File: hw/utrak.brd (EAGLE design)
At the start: 15.9 x 49.8 mm, 46 parts, among them IC1 SI4060, Q1 BLAH, U1 TLV61225

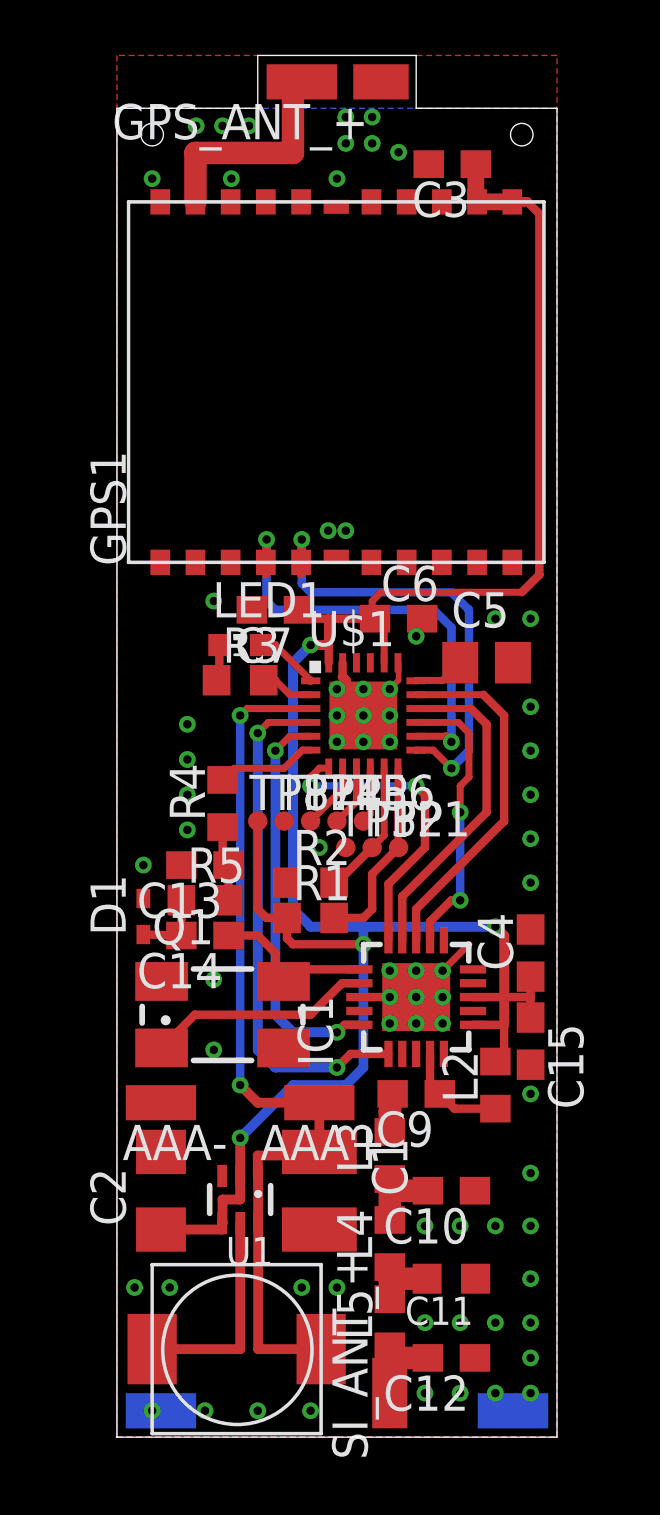
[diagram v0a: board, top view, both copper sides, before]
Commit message: add new hardware files
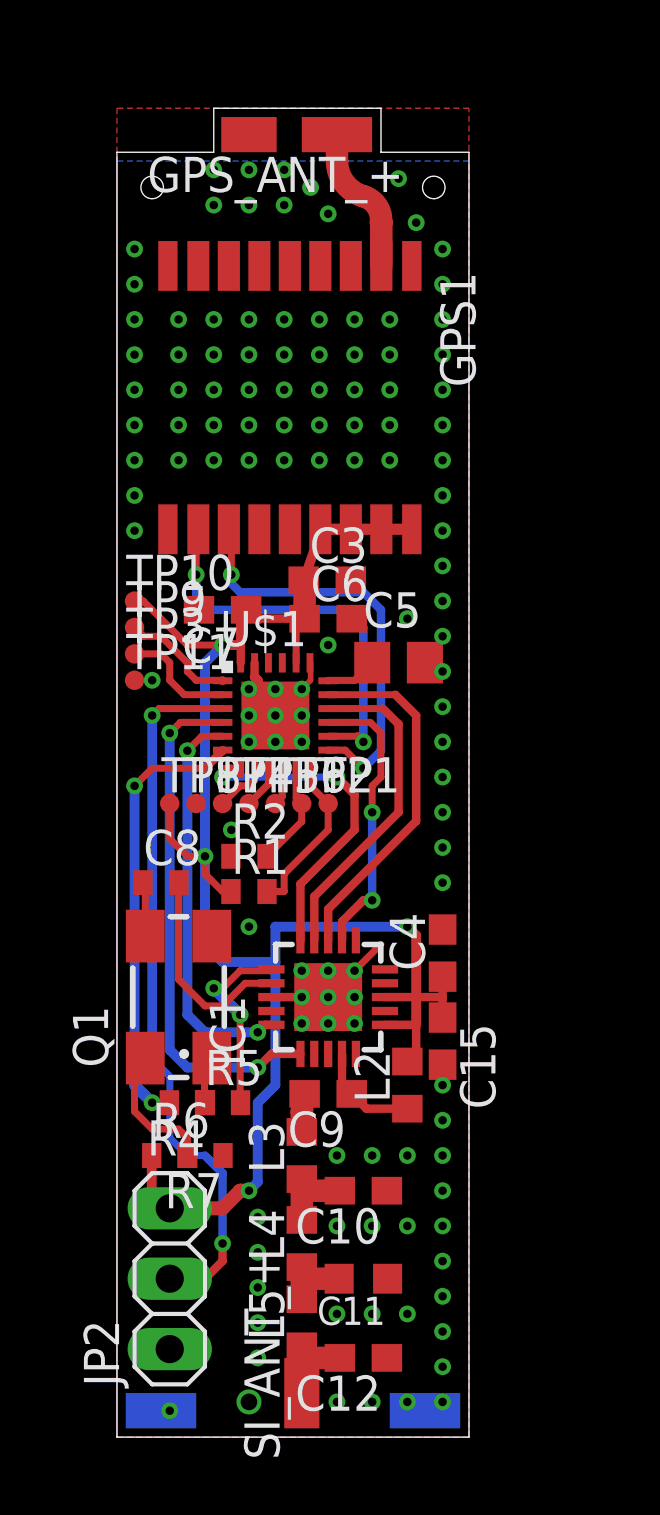
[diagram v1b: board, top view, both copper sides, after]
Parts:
- removed AAA+, AAA-: (no value), wirepad:SMD1,27-2,54
- removed C1: 10u, rcl:C1210
- removed C13: 560p, rcl:C0603
- removed C14: 12p, rcl:C0603
- removed C2: 10u, rcl:C1206
- removed D1: (no value), diode:SOD523
- removed L1: 4u7, l2424:L2424
- removed LED1: (no value), led:SML0603
- removed R3: 470, rcl:R0603
- removed U1: TLV61225, texas_ureg:SC70-6L
- added C8: 8p2, rcl:C0402
- added JP2: (no value), pinhead:1X03
- added R6, R7: 0, rcl:R0402
- added TP10, TP11, TP9: PTR1TP07R, testpad:TP07R
- GPS1: value RXM-GPS-RM-B -> MAX-7; device gps-linx:RXM-GPS-RM-B -> ublox-gps:UBLOX-7
- R1, R2: device rcl:R0603 -> rcl:R0402
- R4: value 220k -> 0; device rcl:R0603 -> rcl:R0402
- R5: value 2M -> 0; device rcl:R0603 -> rcl:R0402
- moved C3 15.7 mm to (7.59, 30.9), turned to 0 degrees
- moved R4 10.9 mm to (2.54, 12.1), turned to 180 degrees
- moved TP3 10.3 mm to (0.64, 28.3)
- moved R5 7.33 mm to (3.81, 12.1)
- moved GPS_ANT_- 5.13 mm to (4.76, 47.0)
- moved TP6 3.24 mm to (5.71, 22.9)
- moved TP4 3.24 mm to (3.81, 22.9)
- moved TP5 3.24 mm to (4.76, 22.9)
- moved TP7 3.24 mm to (2.86, 22.9)
- moved TP8 3.24 mm to (1.91, 22.9)
- moved C5 3.18 mm to (10.2, 27.9)
- moved L2 3.18 mm to (10.5, 12.7)
- moved U$1 3.18 mm to (5.71, 26.0)
- moved C9 3.17 mm to (7.62, 12.4)
- moved IC1 3.17 mm to (7.62, 15.9)
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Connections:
- net XO_MOD renamed XO_EN
- removed net N$1: L1.2, U1.5
- removed net VAAA: AAA+.1, C1.1, L1.1, U$1.3, U1.1, U1.6
- new net ADC_IN: JP2.2, U$1.3
- net +3V3: now also GPS1.6, GPS1.7, GPS1.8, GPS1.9, JP2.3, R6.1, TP10.TP; no longer C2.1, GPS1.11, GPS1.12, U1.2, U1.4
- net GND: now also GPS1.1, GPS1.10, GPS1.12, JP2.1, R7.1, TP11.TP; no longer AAA-.1, C1.2, C13.2, C2.2, D1.A, GPS1.18, GPS1.20, GPS1.21, GPS1.22, Q1.4, TP3.TP, U1.3
- net GPS_ANT_+: now also GPS1.11; no longer GPS1.19
- net GPS_RX: now also GPS1.3; no longer GPS1.5
- net GPS_TX: now also GPS1.2; no longer GPS1.4
- net LED_A: now also TP9.TP; no longer LED1.A
- net LED_K: now also TP3.TP; no longer R3.2
- net N$11: now also Q1.4, R6.2, R7.2; no longer IC1.17, Q1.1
- net N$12: now also C8.1, Q1.3; no longer C14.2, D1.C, R5.1
- net N$13: now also IC1.16; no longer C13.1, R4.1
- net N$14: now also C8.2, IC1.17; no longer C14.1, IC1.16, Q1.3
- net N$8: now also Q1.1, R4.1, R5.1; no longer LED1.C, R3.1
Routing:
- net VAAA: track 32.5 -> 0.00 mm, vias 2 -> 0
- net ADC_IN: track 0.00 -> 25.9 mm, vias 0 -> 2
- net +3V3: track 83.2 -> 65.8 mm
- net XO_EN: track 3.63 -> 16.0 mm, vias 0 -> 2
- net N$1: track 7.72 -> 0.00 mm
- net N$13: track 2.88 -> 6.89 mm, vias 0 -> 2
- net N$11: track 8.10 -> 5.06 mm
- net GPS_ANT_+: track 7.98 -> 5.26 mm
- net LED_K: track 1.91 -> 4.16 mm
- net GPS_TX: track 16.4 -> 14.5 mm
- net GPS_RX: track 17.2 -> 15.3 mm
- net LED_A: track 2.34 -> 4.18 mm
- net N$14: track 6.01 -> 7.58 mm
- net N$3: track 4.94 -> 3.78 mm
- net N$4: track 6.99 -> 6.00 mm
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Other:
- board size 15.9 x 49.8 mm -> 12.7 x 47.9 mm
- board text removed: "uTrak DK3SB"
